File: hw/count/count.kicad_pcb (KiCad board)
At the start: 2 copper layers, 38.4 x 58.9 mm, 19 parts, among them J1 conn_trigger, J2 conn_done, J3 FTDI, J7 Conn_01x01_Male, SW1 reset_count, SW3 switch_reset, U1 ATmega328P-PU, U2 LTC-4724JR, Y1 Crystal

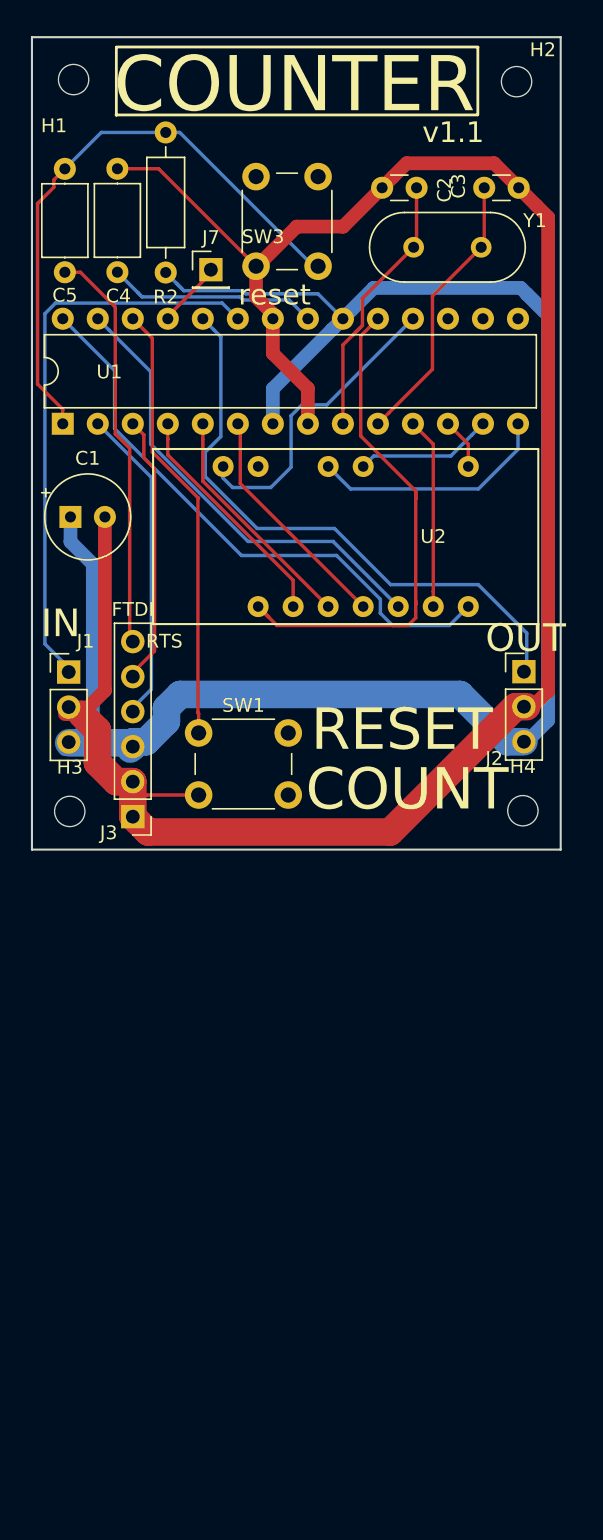
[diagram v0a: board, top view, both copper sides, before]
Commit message: COUNT block v2
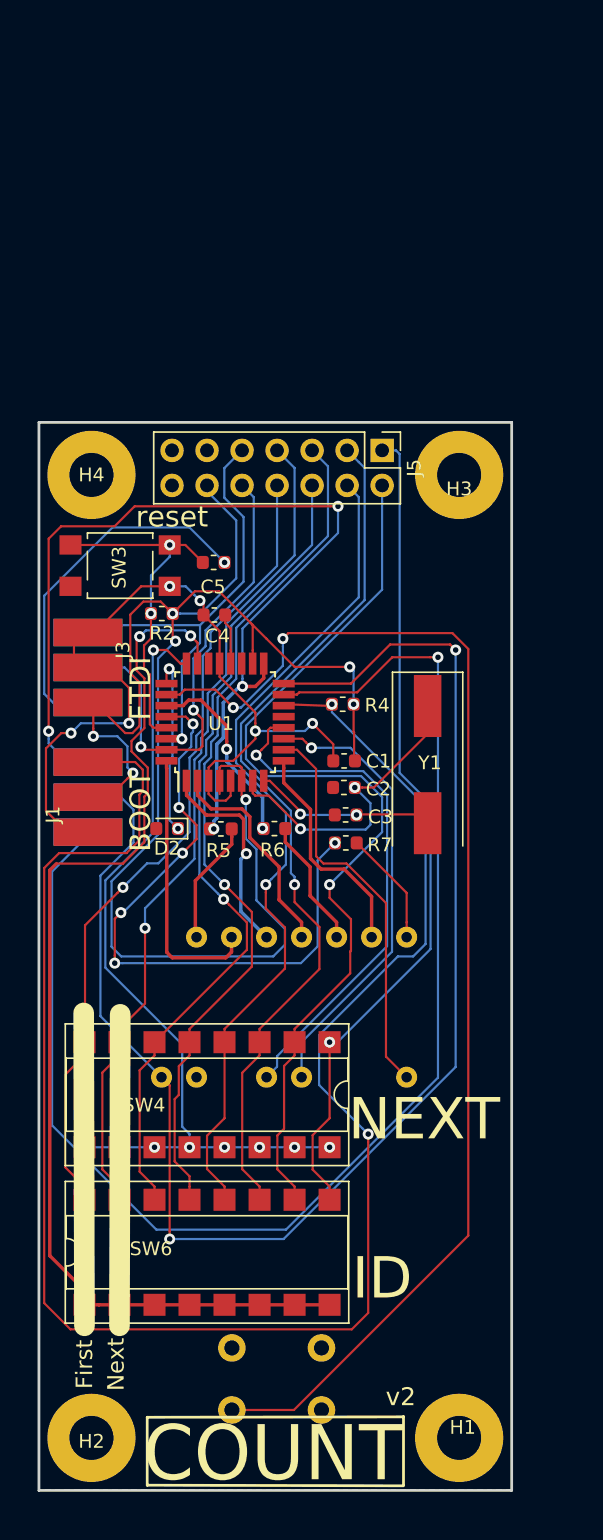
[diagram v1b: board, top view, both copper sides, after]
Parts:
- removed J2: conn_done, Connector_PinHeader_2.54mm:PinHeader_1x03_P2.54mm_Vertical
- removed J7: Conn_01x01_Male, Connector_PinHeader_2.54mm:PinHeader_1x01_P2.54mm_Vertical
- removed SW1: reset_count, autoblocks:SW_PUSH_6mm_H5mm
- added D2: DIODE, Diode_SMD:D_0603_1608Metric, F.Cu at (133.5, 122.4)
- added J5: BUS, Connector_PinHeader_2.54mm:PinHeader_2x07_P2.54mm_Vertical, F.Cu at (149.1, 95.0)
- added R4: 10k, Resistor_SMD:R_0603_1608Metric, F.Cu at (146.2, 113.4)
- added R5: 1k, Resistor_SMD:R_0603_1608Metric, F.Cu at (137.4, 122.5)
- added R6: 1k, Resistor_SMD:R_0603_1608Metric, F.Cu at (141.3, 122.4)
- added R7: 1k, Resistor_SMD:R_0603_1608Metric, F.Cu at (146.5, 123.5)
- added SW2: resetCount, autoblocks:SW_PUSH_6mm_H5mm, B.Cu at (138.2, 164.6)
- added SW4: NEXT, Package_DIP:DIP-16_W7.62mm_SMDSocket_SmallPads, F.Cu at (136.4, 141.7)
- added SW6: ID, Package_DIP:DIP-16_W7.62mm_SMDSocket_SmallPads, F.Cu at (136.4, 153.2)
- C1: footprint Capacitor_THT:CP_Radial_Tantal_D6.0mm_P2.50mm -> Capacitor_SMD:C_0603_1608Metric
- C2, C3: footprint Capacitor_THT:C_Disc_D3.0mm_W1.6mm_P2.50mm -> Capacitor_SMD:C_0603_1608Metric
- C4, C5: footprint Capacitor_THT:C_Axial_L5.1mm_D3.1mm_P7.50mm_Horizontal -> Capacitor_SMD:C_0603_1608Metric
- H1, H2, H3, H4: footprint MountingHole:MountingHole_2.2mm_M2 -> MountingHole:MountingHole_3.2mm_M3_Pad
- J1: value conn_trigger -> bootloader; footprint Connector_PinHeader_2.54mm:PinHeader_1x03_P2.54mm_Vertical -> autoblocks:edge_connector_3
- J3: footprint Connector_PinHeader_2.54mm:PinHeader_1x06_P2.54mm_Vertical -> autoblocks:edge_connector_3
- R2: footprint Resistor_THT:R_Axial_DIN0207_L6.3mm_D2.5mm_P10.16mm_Horizontal -> Resistor_SMD:R_0603_1608Metric
- SW3: value switch_reset -> reset; footprint autoblocks:SW_PUSH_6mm_H5mm -> Button_Switch_SMD:SW_SPST_TL3305C
- U1: value ATmega328P-PU -> ATmega328-AU; footprint Package_DIP:DIP-28_W7.62mm -> Package_QFP:TQFP-32_7x7mm_P0.8mm
- U2: moved to B.Cu
- Y1: footprint Crystal:Crystal_HC18-U_Vertical -> Crystal:Crystal_SMD_HC49-SD
- moved H2 103.1 mm to (128.0, 166.6)
- moved H1 102.4 mm to (154.7, 166.6)
- moved C3 47.2 mm to (146.5, 121.4), turned to 0 degrees
- moved C2 43.6 mm to (146.3, 119.4)
- moved H4 39.7 mm to (128.0, 96.8)
- moved Y1 37.5 mm to (152.4, 117.8), turned to 270 degrees
- moved H3 37.3 mm to (154.7, 96.8)
- moved U2 31.9 mm to (143.3, 134.1)
- moved C5 30.5 mm to (136.9, 103.1), turned to 0 degrees
- moved C1 26.6 mm to (146.3, 117.5), turned to 180 degrees
- moved C4 25.8 mm to (136.9, 106.9), turned to 180 degrees
- moved R2 24.7 mm to (133.1, 106.8), turned to 180 degrees
- moved U1 24.6 mm to (137.7, 114.7)
- moved SW3 23.9 mm to (130.1, 103.4), turned to 180 degrees
- moved J3 12.9 mm to (126.5, 109.5), turned to 270 degrees
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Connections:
- C1 pad 1: VCC -> bus11
- C1 pad 2: GND -> bus13
- C2 pad 1: GND -> bus13
- C3 pad 1: GND -> bus13
- C4 pad 2: GND -> bus13
- J1 pad 1: a0 -> bus13
- J1 pad 2: GND -> bus11
- J1 pad 3: VCC -> d10
- J3 pad 1: GND -> bus13
- J3 pad 2: GND -> bus13
- J3 pad 3: VCC -> bus11
- R2 pad 1: VCC -> bus11
- SW3 pad 1: GND -> bus13
- U1 pad 1: RESET -> d3
- U1 pad 10: XTAL2 -> d6
- U1 pad 11: d5 -> d7
- U1 pad 12: d6 -> d8
- U1 pad 13: d7 -> d9
- U1 pad 14: d8 -> d10
- U1 pad 15: d9 -> d11
- U1 pad 16: d10 -> d12
- U1 pad 17: d11 -> d13
- U1 pad 18: d12 -> bus11
- U1 pad 19: d13 -> Net-(U1-Pad19)
- U1 pad 2: RX -> d4
- U1 pad 20: VCC -> AREF
- U1 pad 21: AREF -> bus13
- U1 pad 22: GND -> Net-(U1-Pad22)
- U1 pad 3: TX -> bus13
- U1 pad 4: d2 -> bus11
- U1 pad 5: d3 -> bus13
- U1 pad 6: d4 -> bus11
- U1 pad 7: VCC -> XTAL1
- U1 pad 8: GND -> XTAL2
- U1 pad 9: XTAL1 -> d5
- U2 pad 1: d13 -> Net-(R5-Pad2)
- U2 pad 5: a4 -> Net-(R6-Pad2)
- U2 pad 7: a5 -> Net-(R7-Pad2)
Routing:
- net GND: track 155.7 -> 0.00 mm
- net d10: track 0.00 -> 132.1 mm, vias 0 -> 2
- net VCC: track 130.1 -> 0.00 mm
- net bus11: track 0.00 -> 126.7 mm, vias 0 -> 7
- net d11: track 0.00 -> 101.0 mm, vias 0 -> 1
- net d12: track 22.1 -> 107.6 mm, vias 0 -> 2
- net bus2: track 0.00 -> 69.1 mm, vias 0 -> 1
- net bus3: track 0.00 -> 63.8 mm, vias 0 -> 1
- net bus13: track 0.00 -> 63.6 mm, vias 0 -> 6
- net bus5: track 0.00 -> 62.7 mm, vias 0 -> 1
- net bus4: track 0.00 -> 61.4 mm, vias 0 -> 1
- net bus7: track 0.00 -> 61.2 mm, vias 0 -> 1
- net bus1: track 0.00 -> 60.8 mm, vias 0 -> 1
- net bus6: track 0.00 -> 60.3 mm, vias 0 -> 1
- net bus8: track 0.00 -> 59.2 mm, vias 0 -> 1
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- added copper zone on B.Cu, net bus11
- added copper zone on F.Cu, net bus13
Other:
- board size 38.4 x 58.9 mm -> 34.3 x 77.5 mm
- rule trace_min: 0.2 -> 0.16
- board text added: "BOOT"
- board text added: "FTDI"
- board text added: "First"
- board text added: "ID"
- board text added: "NEXT"
- board text added: "Next"
- board text added: "RESET COUNT"
- board text added: "v2"
- board text removed: "COUNTER"
- board text removed: "IN"
- board text removed: "OUT"
- board text removed: "RESET"
- board text removed: "RTS"
- board text removed: "v1.1"
